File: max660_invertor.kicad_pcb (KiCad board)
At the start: 2 copper layers, 12 x 17 mm, 5 parts, among them U1 MAX660

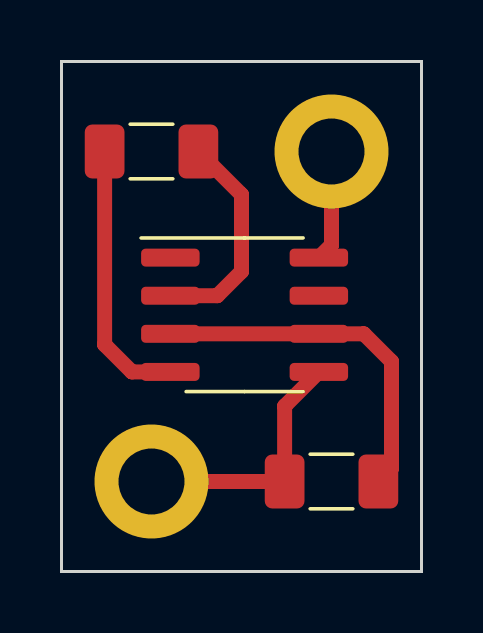
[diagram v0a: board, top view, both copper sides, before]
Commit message: add image
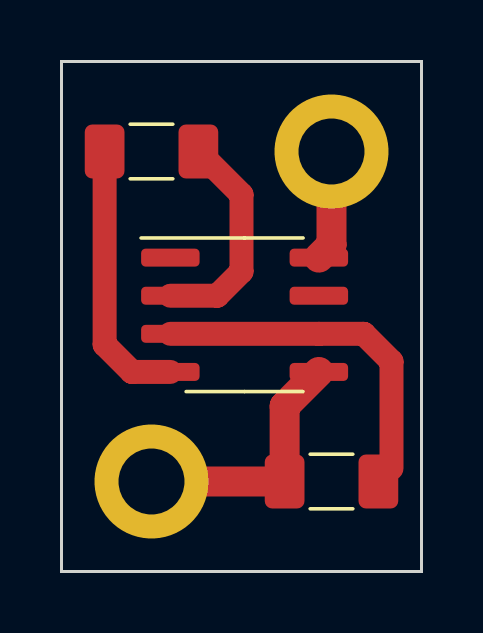
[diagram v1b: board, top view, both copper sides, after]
